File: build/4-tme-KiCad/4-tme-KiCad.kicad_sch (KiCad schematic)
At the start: 29 parts, among them J1 MIDI IN, SW1 RotaryEncoder, SW10 RotaryEncoder, SW11 RotaryEncoder, SW12 RotaryEncoder, SW13 RotaryEncoder, SW14 RotaryEncoder, SW15 RotaryEncoder, SW16 RotaryEncoder, SW2 RotaryEncoder, SW3 RotaryEncoder, SW4 RotaryEncoder, SW5 RotaryEncoder, SW6 RotaryEncoder, SW7 RotaryEncoder, SW8 RotaryEncoder, SW9 RotaryEncoder, U1 CD74HC4067M, U2 CD74HC4067M, U3 6N137

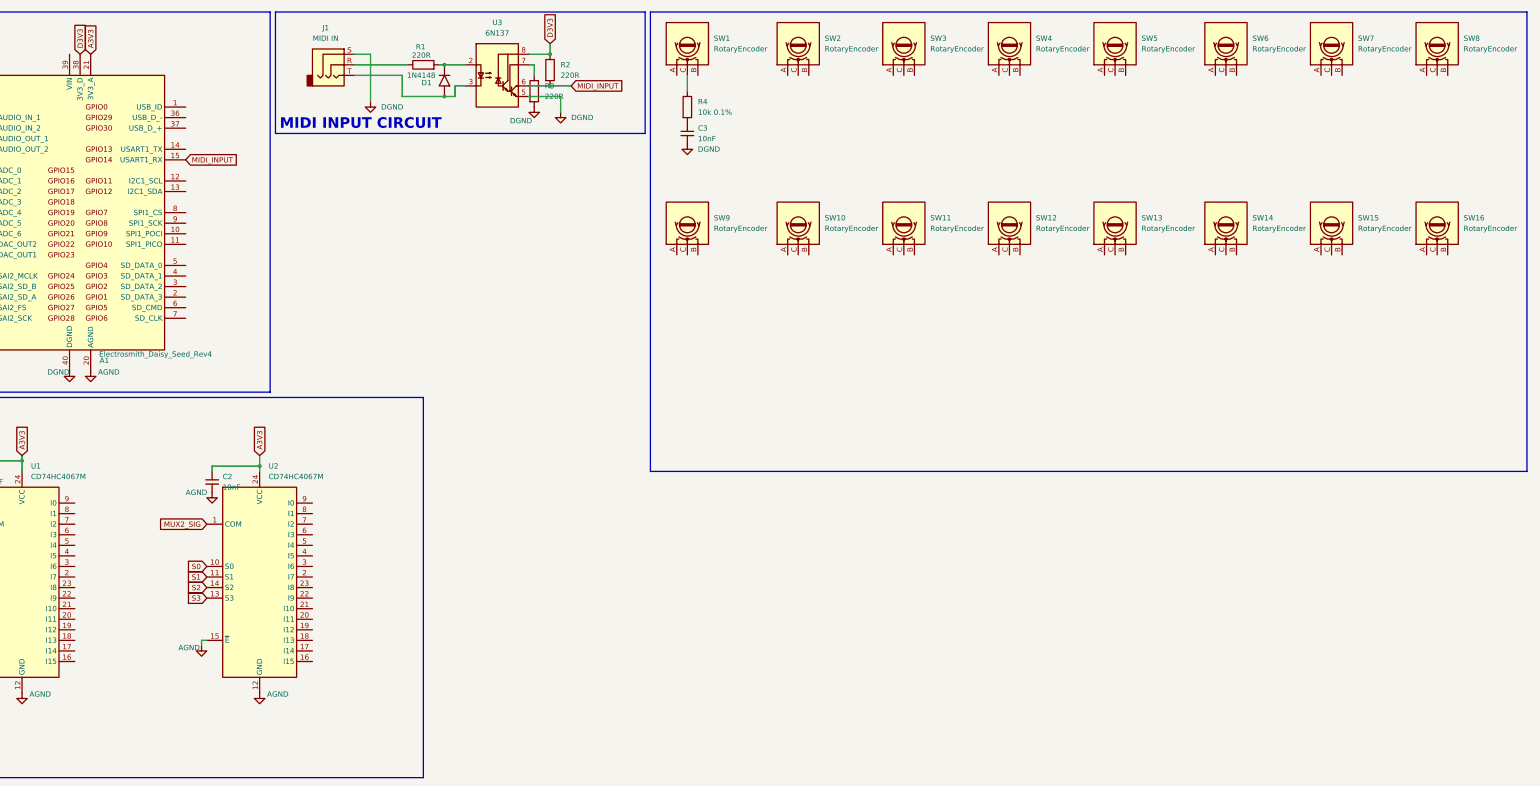
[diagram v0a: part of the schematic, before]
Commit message: REV1
Encoders + MUX
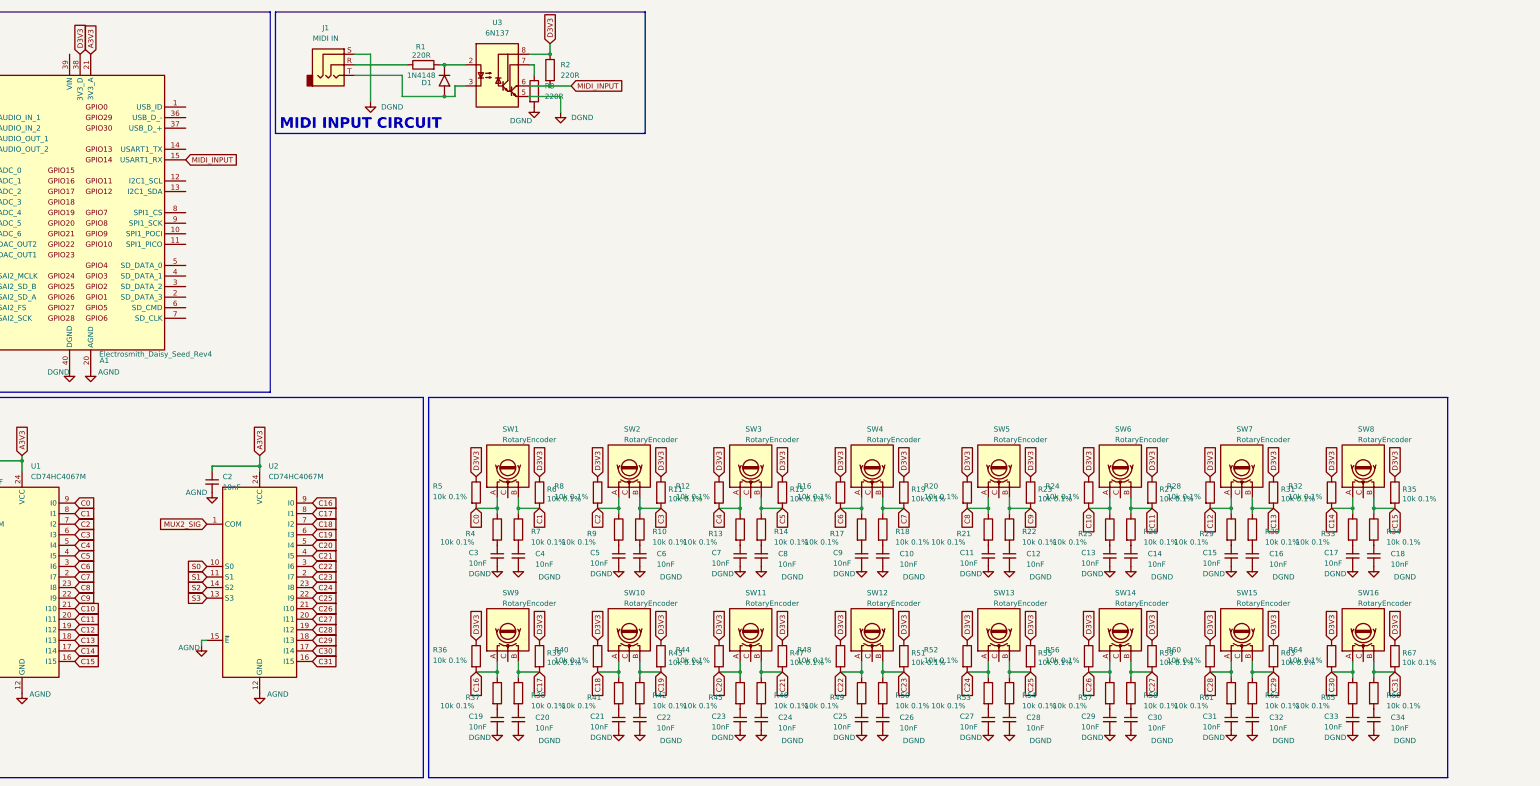
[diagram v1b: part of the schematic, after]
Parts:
- added C10, C11, C12, C13, C14, C15, C16, C17, C18, C19, C20, C21, C22, C23, C24, C25, C26, C27, C28, C29, C30, C31, C32, C33, C34, C4, C5, C6, C7, C8, C9: 10nF_0603_25V, Capacitor_SMD:C_0201_0603Metric, symbol PCM_4ms_Capacitor:10nF_0603_25V
- added R10, R11, R12, R13, R14, R15, R16, R17, R18, R19, R20, R21, R22, R23, R24, R25, R26, R27, R28, R29, R30, R31, R32, R33, R34, R35, R36, R37, R38, R39, R40, R41, R42, R43, R44, R45, R46, R47, R48, R49, R5, R50, R51, R52, R53, R54, R55, R56, R57, R58, R59, R6, R60, R61, R62, R63, R64, R65, R66, R67, R7, R8, R9: 10k_0603_0.1%, 4ms_Resistor:R_0603, symbol PCM_4ms_Resistor:10k_0603_0.1%
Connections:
- net D3V3: now also R11.1, R12.1, R15.1, R16.1, R19.1, R20.1, R23.1, R24.1, R27.1, R28.1, R31.1, R32.1, R35.1, R36.1, R39.1, R40.1, R43.1, R44.1, R47.1, R48.1, R5.1, R51.1, R52.1, R55.1, R56.1, R59.1, R6.1, R60.1, R63.1, R64.1, R67.1, R8.1
- net DGND: now also C10.2, C11.2, C12.2, C13.2, C14.2, C15.2, C16.2, C17.2, C18.2, C19.2, C20.2, C21.2, C22.2, C23.2, C24.2, C25.2, C26.2, C27.2, C28.2, C29.2, C30.2, C31.2, C32.2, C33.2, C34.2, C4.2, C5.2, C6.2, C7.2, C8.2, C9.2
- net C16: now reaches SW9.A
- net C16: now also U2.9 (I0), R36.2, R37.1
- net C17: now reaches SW9.B
- net C17: now also U2.8 (I1), R38.1, R39.2
- net C18: now reaches SW10.A
- net C18: now also U2.7 (I2), R40.2, R41.1
- net C19: now reaches SW10.B
- net C19: now also U2.6 (I3), R42.1, R43.2
- net C8: now reaches SW5.A
- net C8: now also U1.23 (I8), R20.2, R21.1
- net C9: now reaches SW5.B
- net C9: now also U1.22 (I9), R22.1, R23.2
- net C14: now reaches SW8.A
- net C14: now also U1.17 (I14), R32.2, R33.1
- net C15: now reaches SW8.B
- net C15: now also U1.16 (I15), R34.1, R35.2
- net C26: now reaches SW14.A
- net C26: now also U2.21 (I10), R56.2, R57.1
- net C27: now reaches SW14.B
- net C27: now also U2.20 (I11), R58.1, R59.2
- net C22: now reaches SW12.A
- net C22: now also U2.3 (I6), R48.2, R49.1
- net C23: now reaches SW12.B
- net C23: now also U2.2 (I7), R50.1, R51.2
- net C20: now reaches SW11.A
- net C20: now also U2.5 (I4), R44.2, R45.1
- net C21: now reaches SW11.B
- net C21: now also U2.4 (I5), R46.1, R47.2
- net C31: now reaches U2.16 (I15)
- net C31: now also SW16.B, R66.1, R67.2
- net C30: now reaches U2.17 (I14)
- net C30: now also SW16.A, R64.2, R65.1
- net C29: now reaches U2.18 (I13)
- net C29: now also SW15.B, R62.1, R63.2
- net C28: now reaches U2.19 (I12)
- net C28: now also SW15.A, R60.2, R61.1
- net C25: now reaches U2.22 (I9)
- net C25: now also SW13.B, R54.1, R55.2
- net C24: now reaches U2.23 (I8)
- net C24: now also SW13.A, R52.2, R53.1
- net C4: now reaches SW3.A
- net C4: now also U1.5 (I4), R12.2, R13.1
- net C5: now reaches SW3.B
- net C5: now also U1.4 (I5), R14.1, R15.2
- net C10: now reaches SW6.A
- net C10: now also U1.21 (I10), R24.2, R25.1
- net C11: now reaches SW6.B
- net C11: now also U1.20 (I11), R26.1, R27.2
- net C6: now reaches SW4.A
- net C6: now also U1.3 (I6), R16.2, R17.1
- net C7: now reaches SW4.B
- net C7: now also U1.2 (I7), R18.1, R19.2
- net C13: now reaches U1.18 (I13)
- net C13: now also SW7.B, R30.1, R31.2
- net C12: now reaches U1.19 (I12)
- net C12: now also SW7.A, R28.2, R29.1
- net C3: now reaches U1.6 (I3)
- net C3: now also SW2.B, R10.1, R11.2
- net C2: now reaches U1.7 (I2)
- net C2: now also SW2.A, R8.2, R9.1
- net C1: now reaches U1.8 (I1)
- net C1: now also SW1.B, R6.2, R7.1
- net C0: now reaches U1.9 (I0)
- net C0: now also R4.1, SW1.A, R5.2
- net at SW1.C: no longer R4.1
- new net: C8.1, R14.2
- new net: C29.1, R57.2
- new net: C27.1, R53.2
- new net: C24.1, R46.2
- new net: C21.1, R41.2
- new net: C9.1, R17.2
- new net: C26.1, R50.2
- new net: C4.1, R7.2
- new net: C30.1, R58.2
- new net: C6.1, R10.2
- new net: C15.1, R29.2
- new net: C14.1, R26.2
- new net: C20.1, R38.2
- new net: C16.1, R30.2
- new net: C5.1, R9.2
- new net: C11.1, R21.2
- new net: C7.1, R13.2
- new net: C28.1, R54.2
- new net: C25.1, R49.2
- new net: C22.1, R42.2
- new net: C23.1, R45.2
- new net: C18.1, R34.2
- new net: C13.1, R25.2
- new net: C34.1, R66.2
- new net: C12.1, R22.2
- new net: C10.1, R18.2
- new net: C33.1, R65.2
- new net: C31.1, R61.2
- new net: C32.1, R62.2
- new net: C17.1, R33.2
- new net: C19.1, R37.2
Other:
- moved on the sheet: C3, R4, SW1

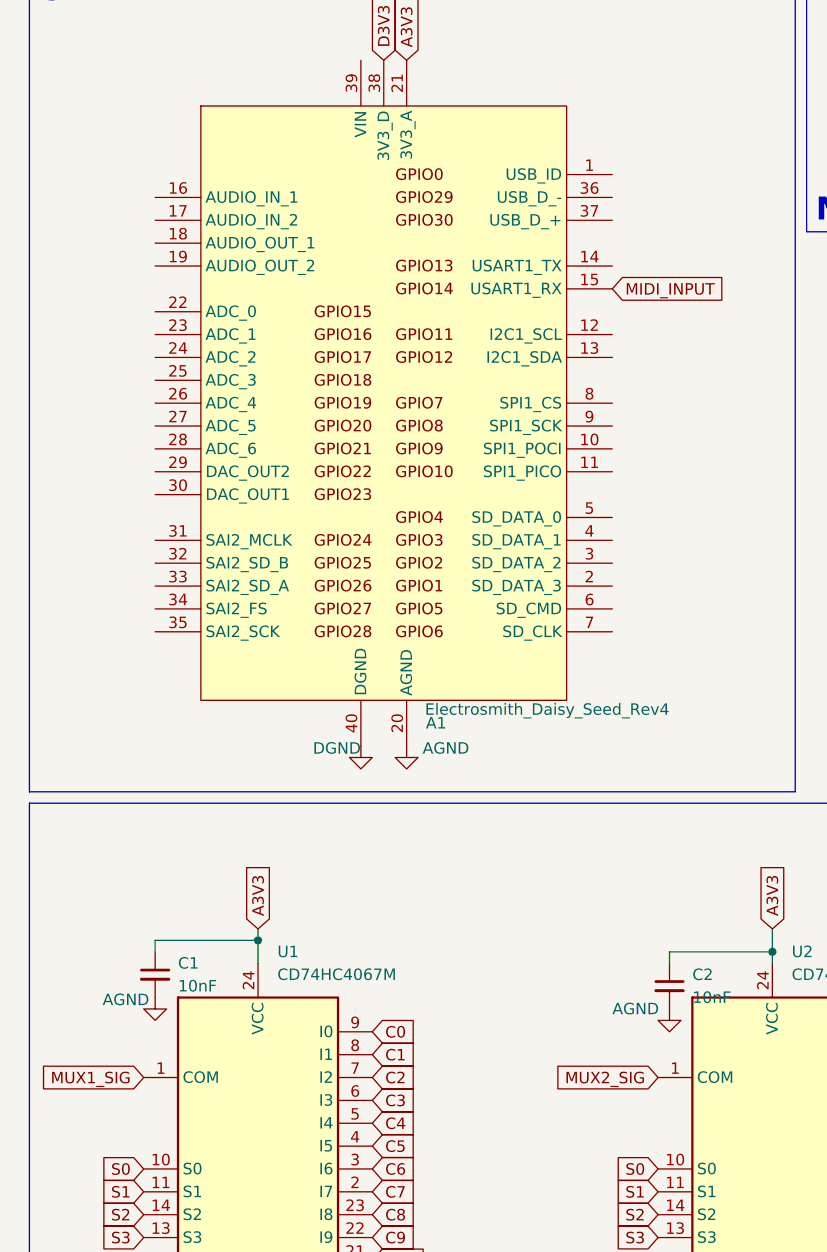
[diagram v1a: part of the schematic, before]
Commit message: Update 4-tme-KiCad.kicad_sch
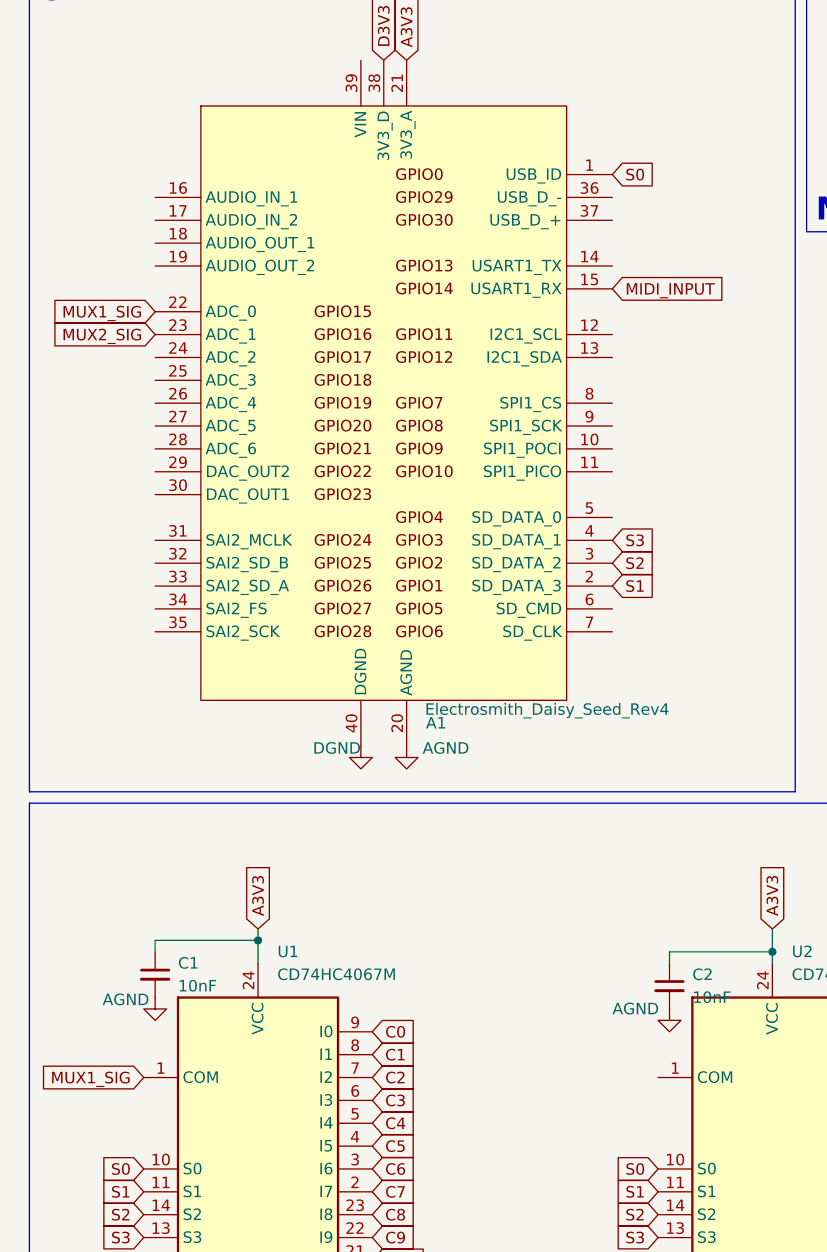
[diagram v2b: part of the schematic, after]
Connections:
- net MUX1_SIG: now also A1.22 (ADC_0)
- net MUX2_SIG: now also A1.23 (ADC_1); no longer U2.1 (COM)
- net S0: now also A1.1 (USB_ID)
- net S1: now also A1.2 (SD_DATA_3)
- net S2: now also A1.3 (SD_DATA_2)
- net S3: now also A1.4 (SD_DATA_1)

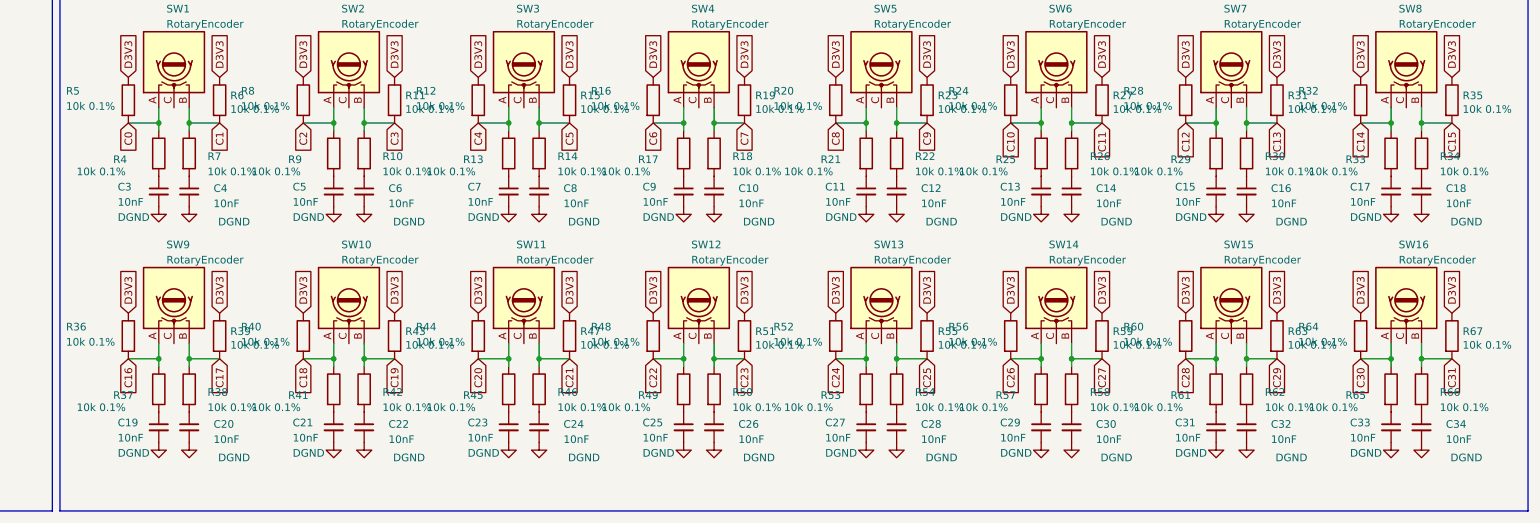
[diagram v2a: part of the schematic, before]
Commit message: rev1
encoders revision 3
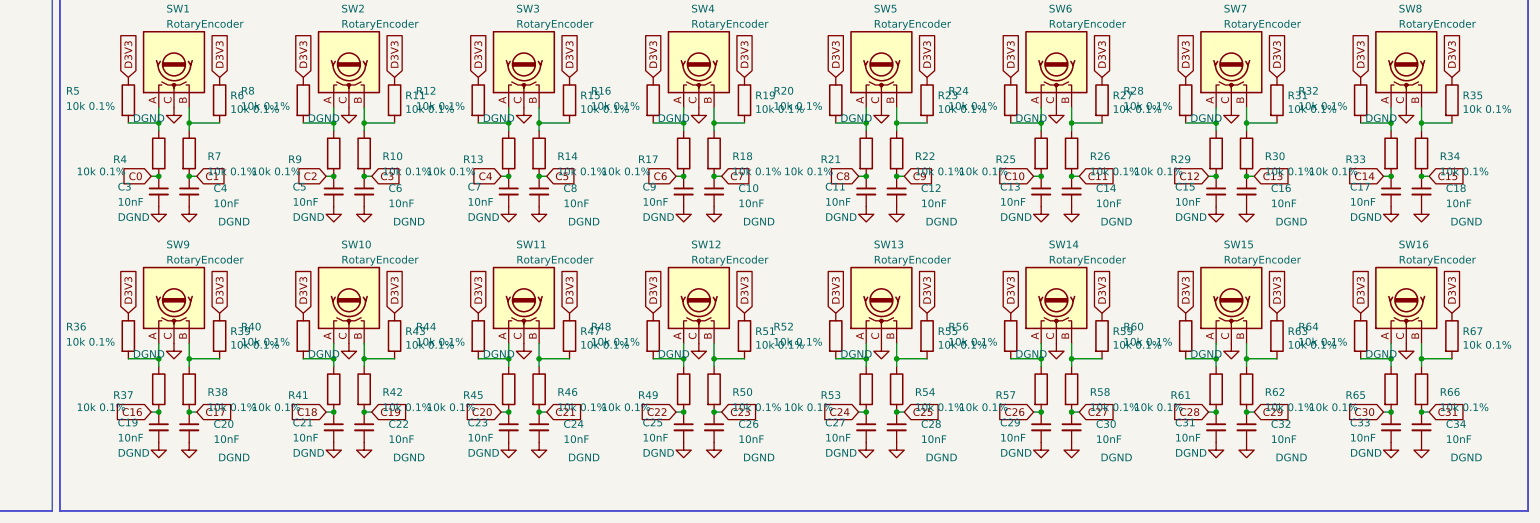
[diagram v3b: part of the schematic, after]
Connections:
- net C0: now also C3.1, R4.2; no longer R4.1, R5.2, SW1.A
- net C1: now also C4.1, R7.2; no longer R6.2, R7.1, SW1.B
- net C10: now also C13.1, R25.2; no longer R24.2, R25.1, SW6.A
- net C11: now also C14.1, R26.2; no longer R26.1, R27.2, SW6.B
- net C12: now also C15.1, R29.2; no longer R28.2, R29.1, SW7.A
- net C13: now also C16.1, R30.2; no longer R30.1, R31.2, SW7.B
- net C14: now also C17.1, R33.2; no longer R32.2, R33.1, SW8.A
- net C15: now also C18.1, R34.2; no longer R34.1, R35.2, SW8.B
- net C16: now also C19.1, R37.2; no longer R36.2, R37.1, SW9.A
- net C17: now also C20.1, R38.2; no longer R38.1, R39.2, SW9.B
- net C18: now also C21.1, R41.2; no longer R40.2, R41.1, SW10.A
- net C19: now also C22.1, R42.2; no longer R42.1, R43.2, SW10.B
- net C2: now also C5.1, R9.2; no longer R8.2, R9.1, SW2.A
- net C20: now also C23.1, R45.2; no longer R44.2, R45.1, SW11.A
- net C21: now also C24.1, R46.2; no longer R46.1, R47.2, SW11.B
- net C22: now also C25.1, R49.2; no longer R48.2, R49.1, SW12.A
- net C23: now also C26.1, R50.2; no longer R50.1, R51.2, SW12.B
- net C24: now also C27.1, R53.2; no longer R52.2, R53.1, SW13.A
- net C25: now also C28.1, R54.2; no longer R54.1, R55.2, SW13.B
- net C26: now also C29.1, R57.2; no longer R56.2, R57.1, SW14.A
- net C27: now also C30.1, R58.2; no longer R58.1, R59.2, SW14.B
- net C28: now also C31.1, R61.2; no longer R60.2, R61.1, SW15.A
- net C29: now also C32.1, R62.2; no longer R62.1, R63.2, SW15.B
- net C3: now also C6.1, R10.2; no longer R10.1, R11.2, SW2.B
- net C30: now also C33.1, R65.2; no longer R64.2, R65.1, SW16.A
- net C31: now also C34.1, R66.2; no longer R66.1, R67.2, SW16.B
- net C4: now also C7.1, R13.2; no longer R12.2, R13.1, SW3.A
- net C5: now also C8.1, R14.2; no longer R14.1, R15.2, SW3.B
- net C6: now also C9.1, R17.2; no longer R16.2, R17.1, SW4.A
- net C7: now also C10.1, R18.2; no longer R18.1, R19.2, SW4.B
- net C8: now also C11.1, R21.2; no longer R20.2, R21.1, SW5.A
- net C9: now also C12.1, R22.2; no longer R22.1, R23.2, SW5.B
- net DGND: now also SW1.C, SW10.C, SW11.C, SW12.C, SW13.C, SW14.C, SW15.C, SW16.C, SW2.C, SW3.C, SW4.C, SW5.C, SW6.C, SW7.C, SW8.C, SW9.C
- new net: R16.2, R17.1, SW4.A
- new net: R62.1, R63.2, SW15.B
- new net: R34.1, R35.2, SW8.B
- new net: R46.1, R47.2, SW11.B
- new net: R40.2, R41.1, SW10.A
- new net: R50.1, R51.2, SW12.B
- new net: R52.2, R53.1, SW13.A
- new net: R54.1, R55.2, SW13.B
- new net: R58.1, R59.2, SW14.B
- new net: R36.2, R37.1, SW9.A
- new net: R38.1, R39.2, SW9.B
- new net: R10.1, R11.2, SW2.B
- new net: R56.2, R57.1, SW14.A
- new net: R28.2, R29.1, SW7.A
- new net: R60.2, R61.1, SW15.A
- new net: R30.1, R31.2, SW7.B
- new net: R32.2, R33.1, SW8.A
- new net: R48.2, R49.1, SW12.A
- new net: R8.2, R9.1, SW2.A
- new net: R6.2, R7.1, SW1.B
- new net: R12.2, R13.1, SW3.A
- new net: R64.2, R65.1, SW16.A
- new net: R66.1, R67.2, SW16.B
- new net: R4.1, R5.2, SW1.A
- new net: R18.1, R19.2, SW4.B
- new net: R26.1, R27.2, SW6.B
- new net: R44.2, R45.1, SW11.A
- new net: R20.2, R21.1, SW5.A
- new net: R22.1, R23.2, SW5.B
- new net: R24.2, R25.1, SW6.A
- new net: R14.1, R15.2, SW3.B
- new net: R42.1, R43.2, SW10.B
